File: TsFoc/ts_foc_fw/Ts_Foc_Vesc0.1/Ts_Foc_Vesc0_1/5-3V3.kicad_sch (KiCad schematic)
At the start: 5 parts, among them U2 AMS1117-3.3V

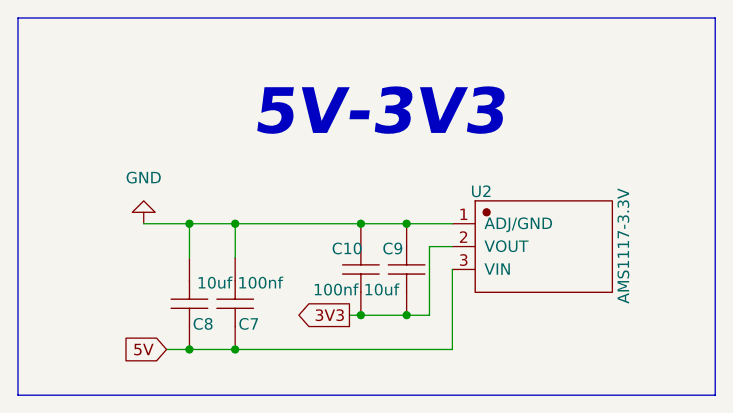
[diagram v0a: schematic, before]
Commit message: 同步_Tue Feb  4 22:38:42     2025
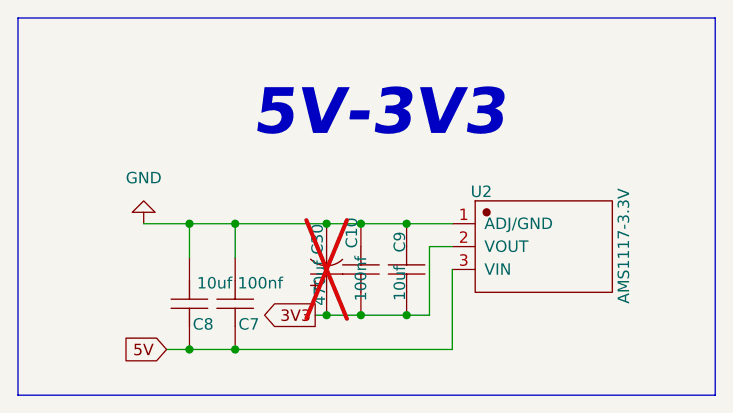
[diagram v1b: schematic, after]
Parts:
- added C30: 470uf, Ts_Foc_Vo封装库:Cap_Electrolytic, symbol Ts_Foc_Vo符号库:Cap_Electrolytic
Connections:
- net 3V3: now also C30.1
- net GND: now also C30.2
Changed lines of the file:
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@@
+	)
+	(junction
+		(at 241.3 35.56)
+		(diameter 0)
+		(color 0 0 0 0)
 	)
 	(junction
@@
 	)
 	(junction
+		(at 241.3 45.72)
+		(diameter 0)
+		(color 0 0 0 0)
+	)
+	(junction
 		(at 245.11 45.72)
 		(diameter 0)
@@
 	(wire
 		(pts
-			(xy 231.14 35.56) (xy 245.11 35.56)
+			(xy 231.14 35.56) (xy 241.3 35.56)
 		)
 		(stroke
@@
 	(wire
 		(pts
-			(xy 243.84 45.72) (xy 245.11 45.72)
+			(xy 240.03 45.72) (xy 241.3 45.72)
 		)
 		(stroke
@@
 	(wire
 		(pts
+			(xy 241.3 35.56) (xy 245.11 35.56)
+		)
+		(stroke
+			(width 0)
+			(type default)
+		)
+	)
+	(wire
+		(pts
 			(xy 223.52 49.53) (xy 226.06 49.53)
 		)
@@
 		(pts
 			(xy 250.19 45.72) (xy 252.73 45.72)
+		)
+		(stroke
+			(width 0)
+			(type default)
+		)
+	)
+	(wire
+		(pts
+			(xy 241.3 45.72) (xy 245.11 45.72)
 		)
 		(stroke
@@
 	(global_label "3V3"
 		(shape output)
-		(at 243.84 45.72 180)
+		(at 240.03 45.72 180)
 		(fields_autoplaced yes)
 		(effects
@@
 		)
 		(property "Intersheetrefs" "${INTERSHEET_REFS}"
-			(at 237.3472 45.72 0)
+			(at 233.5372 45.72 0)
 			(effects
 				(font
@@
 		(dnp no)
 		(property "Reference" "C10"
-			(at 243.586 38.354 90)
+			(at 244.094 36.576 0)
 			(effects
 				(font
@@
 		)
 		(property "Value" "100nf"
-			(at 242.316 42.926 90)
+			(at 245.11 41.656 0)
 			(effects
 				(font
@@
 		(dnp no)
 		(property "Reference" "C9"
-			(at 248.666 38.354 90)
+			(at 249.428 37.592 0)
 			(effects
 				(font
@@
 		)
 		(property "Value" "10uf"
-			(at 247.396 42.926 90)
+			(at 249.428 42.164 0)
 			(effects
 				(font
@@
 					(unit 1)
 				)
+			)
+		)
+	)
+	(symbol
+		(lib_id "Ts_Foc_Vo符号库:Cap_Electrolytic")
+		(at 241.3 40.64 90)
+		(unit 1)
+		(exclude_from_sim yes)
+		(in_bom no)
+		(on_board no)
+		(dnp yes)
+		(property "Reference" "C30"
+			(at 240.284 35.56 0)
+			(effects
+				(font
+					(size 1.27 1.27)
+				)
+				(justify right)
+			)
+		)
+		(property "Value" "470uf"
+			(at 240.538 39.624 0)
+			(effects
+				(font
+					(size 1.27 1.27)
+				)
+				(justify right)
+			)
+		)
+		(property "Footprint" "Ts_Foc_Vo封装库:Cap_Electrolytic"
+			(at 244.094 40.386 0)
+			(effects
+				(font
+					(size 1.27 1.27)
+				)
+				(hide yes)
+			)
+		)
+		(property "Datasheet" ""
+			(at 247.142 40.64 0)
+			(effects
+				(font
+					(size 1.27 1.27)
+				)
+				(hide yes)
+			)
+		)
+		(property "Description" ""
+			(at 241.3 40.64 0)
+			(effects
+				(font
+					(size 1.27 1.27)
+				)
+				(hide yes)
+			)
+		)
+		(property "SuppliersPartNumber" "C2960233"
+			(at 244.094 40.894 0)
+			(effects
+				(font
+					(size 1.27 1.27)
+				)
+				(hide yes)
+			)
+		)
+		(property "uuid" "std:f2c4c4acb06341a6b501ff67d9191846"
+			(at 244.094 40.894 0)
+			(effects
+				(font
+					(size 1.27 1.27)
+				)
+				(hide yes)
+			)
+		)
+		(pin "2"
+		)
+		(pin "1"
+		)
+		(instances
+			(project "Ts_Foc_Vo1_0"
+				(path "/0cbcabec-8024-48c7-ab91-86e279a5637e/97ee4039-d600-4608-b2ff-7d42036ea92c/e8a44f51-cbda-485e-b097-3ee1dbcae92f"
+					(reference "C30")
+					(unit 1)
+				)
